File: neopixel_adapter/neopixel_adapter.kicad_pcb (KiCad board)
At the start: 2 copper layers, 15.2 x 5.1 mm, 5 parts, among them J1 Conn_01x02, J2 Conn_01x02

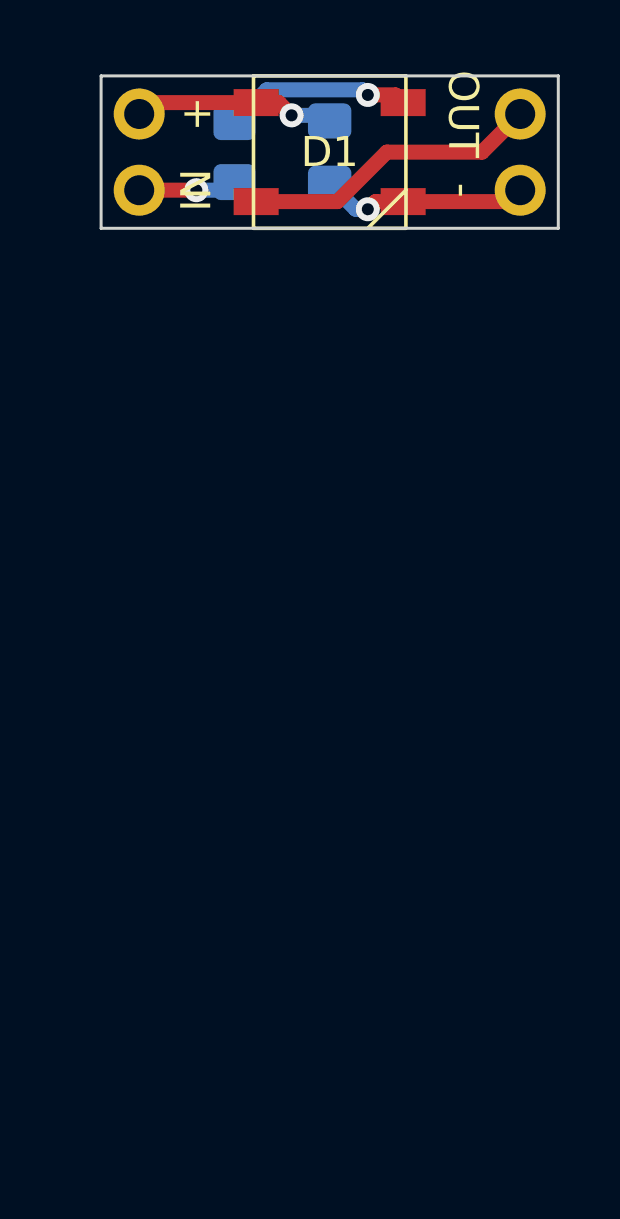
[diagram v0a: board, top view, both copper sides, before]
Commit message: Add .gitignore.
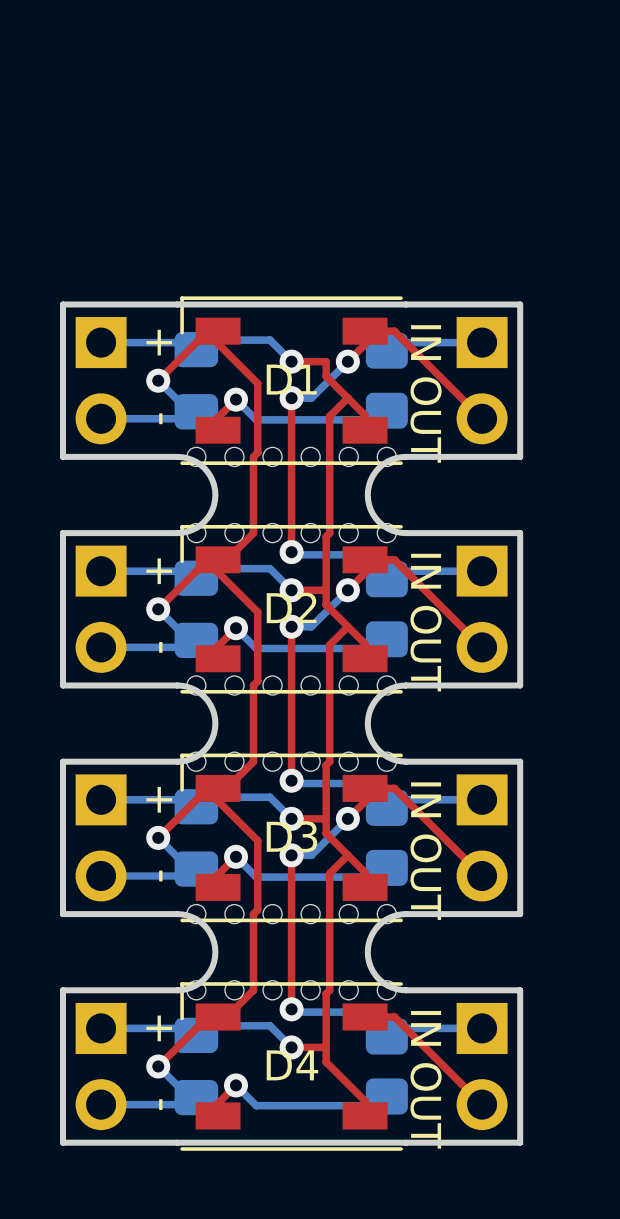
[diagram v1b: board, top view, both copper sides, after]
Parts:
- added C2: 0.1uF, Capacitor_SMD:C_0805_2012Metric_Pad1.18x1.45mm_HandSolder, B.Cu at (131.4, 83.8)
- added C3: 0.1uF, Capacitor_SMD:C_0805_2012Metric_Pad1.18x1.45mm_HandSolder, B.Cu at (131.4, 91.4)
- added C4: 0.1uF, Capacitor_SMD:C_0805_2012Metric_Pad1.18x1.45mm_HandSolder, B.Cu at (131.4, 99.1)
- added D2: WS2812B, LED_SMD:LED_WS2812B_PLCC4_5.0x5.0mm_P3.2mm, F.Cu at (134.6, 83.8)
- added D3: WS2812B, LED_SMD:LED_WS2812B_PLCC4_5.0x5.0mm_P3.2mm, F.Cu at (134.6, 91.4)
- added D4: WS2812B, LED_SMD:LED_WS2812B_PLCC4_5.0x5.0mm_P3.2mm, F.Cu at (134.6, 99.1)
- added J3: Conn_01x02, Connector_PinHeader_2.54mm:PinHeader_1x02_P2.54mm_Vertical, B.Cu at (128.3, 82.5)
- added J4: Conn_01x02, Connector_PinHeader_2.54mm:PinHeader_1x02_P2.54mm_Vertical, B.Cu at (141.0, 82.5)
- added J5: Conn_01x02, Connector_PinHeader_2.54mm:PinHeader_1x02_P2.54mm_Vertical, B.Cu at (128.3, 90.2)
- added J6: Conn_01x02, Connector_PinHeader_2.54mm:PinHeader_1x02_P2.54mm_Vertical, B.Cu at (141.0, 90.2)
- added J7: Conn_01x02, Connector_PinHeader_2.54mm:PinHeader_1x02_P2.54mm_Vertical, B.Cu at (128.3, 97.8)
- added J8: Conn_01x02, Connector_PinHeader_2.54mm:PinHeader_1x02_P2.54mm_Vertical, B.Cu at (141.0, 97.8)
- added R2: 470R, Resistor_SMD:R_0805_2012Metric_Pad1.20x1.40mm_HandSolder, B.Cu at (137.8, 83.8)
- added R3: 470R, Resistor_SMD:R_0805_2012Metric_Pad1.20x1.40mm_HandSolder, B.Cu at (137.8, 91.4)
- added R4: 470R, Resistor_SMD:R_0805_2012Metric_Pad1.20x1.40mm_HandSolder, B.Cu at (137.8, 99.1)
- added REF**: Mouse_Bites_0.2in, Custom:Mouse_Bites_0.2in, F.Cu at (134.6, 87.6)
- added REF**: Mouse_Bites_0.2in, Custom:Mouse_Bites_0.2in, F.Cu at (134.6, 80.0)
- added REF**: Mouse_Bites_0.2in, Custom:Mouse_Bites_0.2in, F.Cu at (134.6, 95.2)
- moved R1 9.16 mm to (137.8, 76.2), turned to -90 degrees
- moved C1 8.82 mm to (131.4, 76.2), turned to 90 degrees
- moved J2 7.73 mm to (141.0, 74.9)
- moved D1 7.73 mm to (134.6, 76.2), turned to 180 degrees
- moved J1 7.73 mm to (128.3, 74.9)
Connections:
- C1 pad 1: /VDD -> /NeoPixel Module 1/VSS
- C1 pad 2: /VSS -> /NeoPixel Module 1/VDD
- D1 pad 1: /VDD -> /NeoPixel Module 1/VDD
- D1 pad 2: /DOUT -> /NeoPixel Module 1/DOUT
- D1 pad 3: /VSS -> /NeoPixel Module 1/VSS
- J1 pad 1: /VDD -> /NeoPixel Module 1/VDD
- J1 pad 2: /DIN -> /NeoPixel Module 1/VSS
- J2 pad 1: /DOUT -> /NeoPixel Module 1/DIN
- J2 pad 2: /VSS -> /NeoPixel Module 1/DOUT
- R1 pad 1: /DIN -> /NeoPixel Module 1/DIN
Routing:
- net /NeoPixel Module 1/VDD: track 0.00 -> 63.5 mm, vias 0 -> 4
- net /NeoPixel Module 1/VSS: track 0.00 -> 57.3 mm, vias 0 -> 4
- net /NeoPixel Module 1/DOUT: track 0.00 -> 20.7 mm, vias 0 -> 3
- net /NeoPixel Module 2/DOUT: track 0.00 -> 20.7 mm, vias 0 -> 3
- net /NeoPixel Module 3/DOUT: track 0.00 -> 20.7 mm, vias 0 -> 3
- net /DOUT: track 10.0 -> 0.00 mm
- net /VSS: track 6.97 -> 0.00 mm, vias 1 -> 0
- net /VDD: track 6.76 -> 0.00 mm, vias 1 -> 0
- net Net-(D2-DIN): track 0.00 -> 6.70 mm, vias 0 -> 1
- net Net-(D3-DIN): track 0.00 -> 6.70 mm, vias 0 -> 1
- net Net-(D4-DIN): track 0.00 -> 6.70 mm, vias 0 -> 1
- net /NeoPixel Module 4/DOUT: track 0.00 -> 5.11 mm
- net /NeoPixel Module 1/DIN: track 0.00 -> 3.29 mm
- net /DIN: track 3.29 -> 0.00 mm, vias 1 -> 0
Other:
- board size 15.2 x 5.1 mm -> 15.2 x 27.9 mm
